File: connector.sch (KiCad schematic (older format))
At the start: 2 parts, among them J11 Conn_02x05_Counter_Clockwise, J12 DB9_Male_MountingHoles

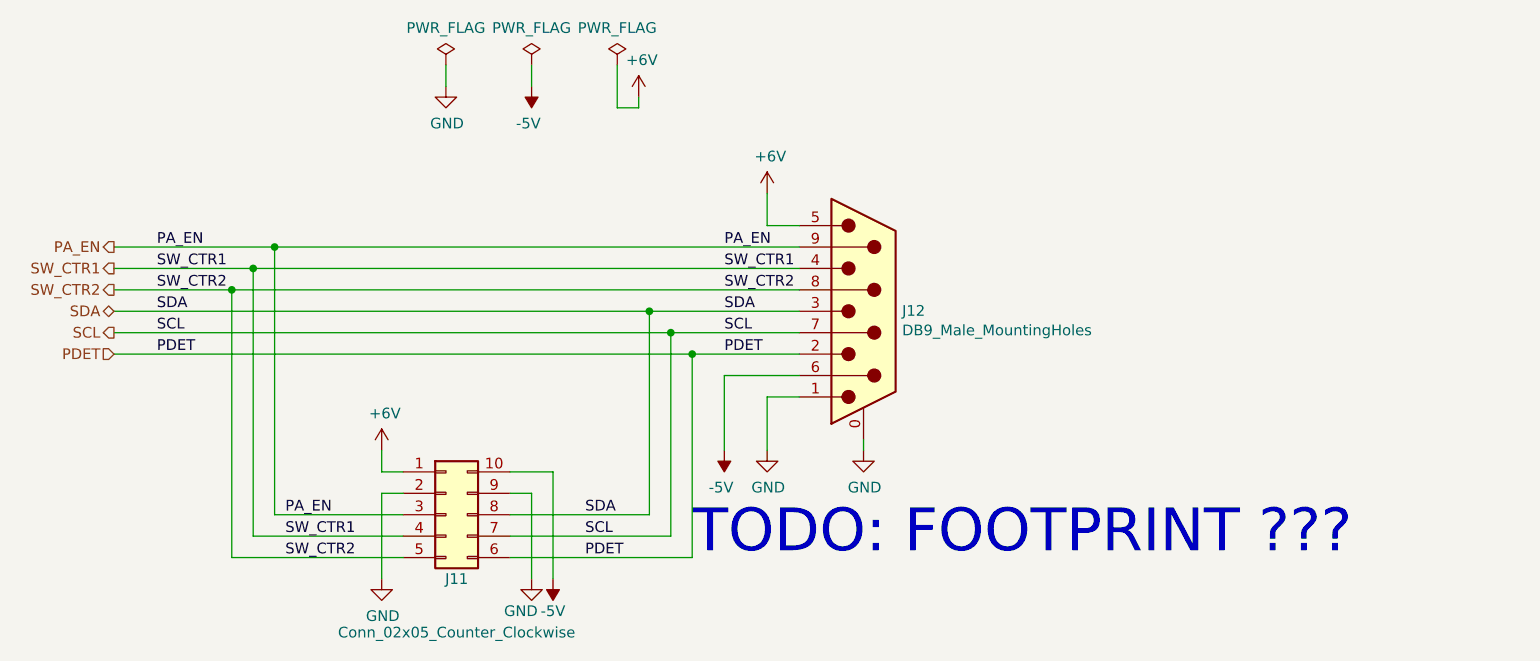
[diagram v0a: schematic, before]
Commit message: First layout
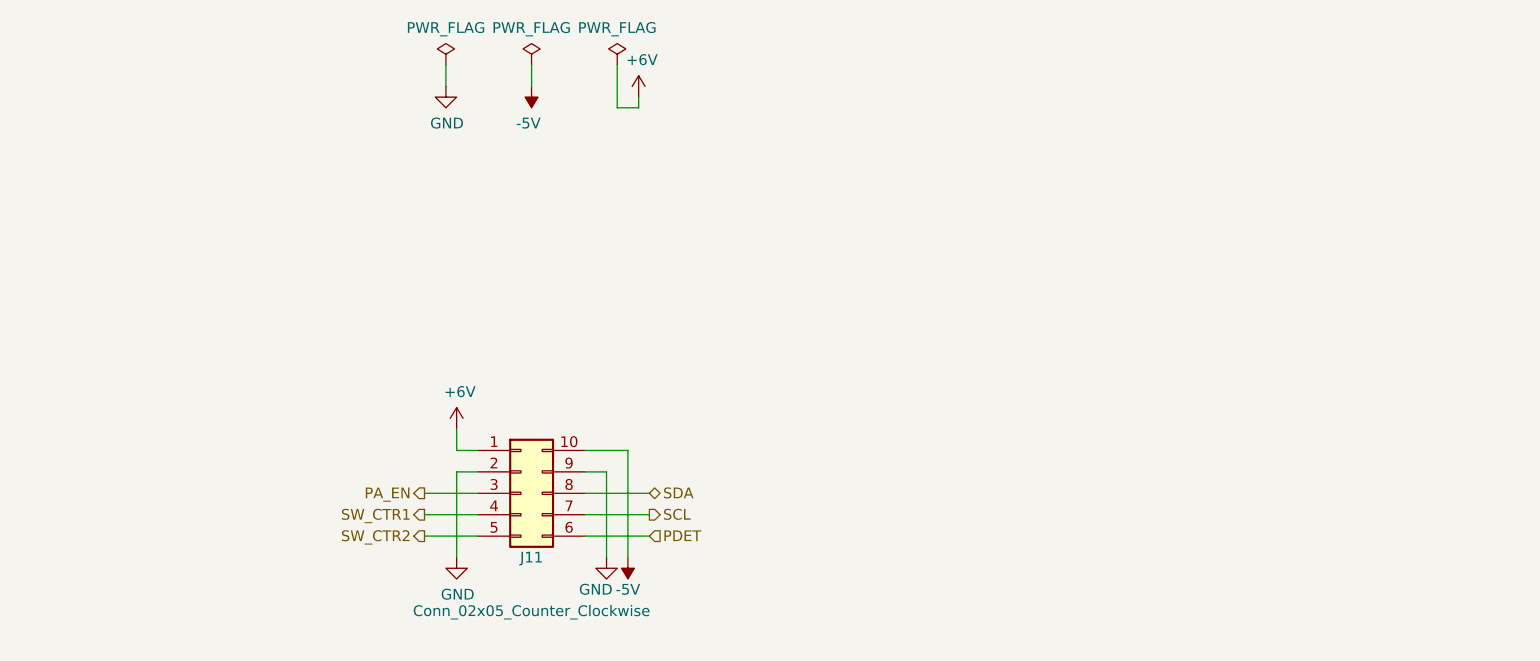
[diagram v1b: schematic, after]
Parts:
- removed J12: DB9_Male_MountingHoles, symbol Connector:DB9_Male_MountingHoles
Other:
- note removed: "TODO: FOOTPRINT ???\n"
- moved on the sheet: J11

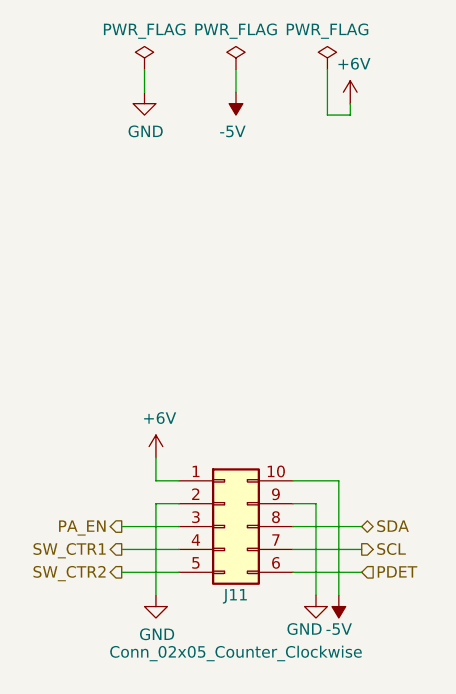
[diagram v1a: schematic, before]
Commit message: Fixed connector
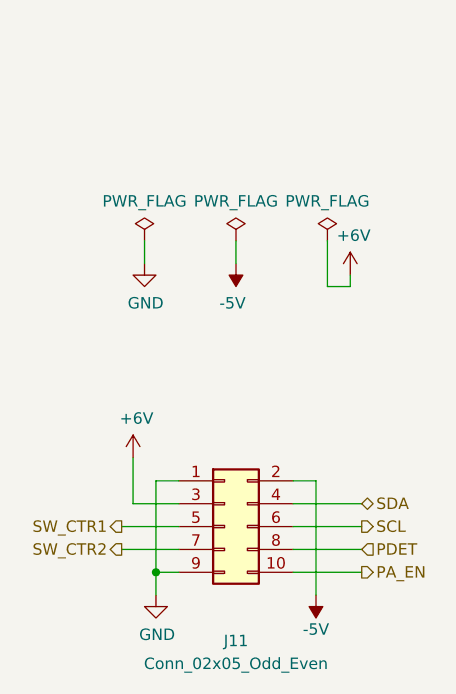
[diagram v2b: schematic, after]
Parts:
- removed J11: Conn_02x05_Counter_Clockwise, Connector_IDC:IDC-Header_2x05_P2.54mm_Vertical, symbol Connector_Generic:Conn_02x05_Counter_Clockwise
- added J11: Conn_02x05_Odd_Even, Connector_IDC:IDC-Header_2x05_P2.54mm_Vertical, symbol Connector_Generic:Conn_02x05_Odd_Even
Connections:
- net +6V: now also J11.3 (Pin_3)
- net -5V: now also J11.2 (Pin_2)
- net GND: now also J11.1 (Pin_1), J11.9 (Pin_9)
- net PA_EN: now also J11.10 (Pin_10)
- net PDET: now also J11.8 (Pin_8)
- net SCL: now also J11.6 (Pin_6)
- net SDA: now also J11.4 (Pin_4)
- net SW_CTR1: now also J11.5 (Pin_5)
- net SW_CTR2: now also J11.7 (Pin_7)
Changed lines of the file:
@@
 Comment4 ""
 $EndDescr
+Text HLabel 6300 4450 2    50   Output ~ 0
+PA_EN
 Text HLabel 5250 4250 0    50   Output ~ 0
-PA_EN
+SW_CTR1
 Text HLabel 5250 4350 0    50   Output ~ 0
-SW_CTR1
-Text HLabel 5250 4450 0    50   Output ~ 0
 SW_CTR2
-Text HLabel 6300 4250 2    50   BiDi ~ 0
+Text HLabel 6300 4150 2    50   BiDi ~ 0
 SDA
-Text HLabel 6300 4350 2    50   Output ~ 0
+Text HLabel 6300 4250 2    50   Output ~ 0
 SCL
-Text HLabel 6300 4450 2    50   Input ~ 0
+Text HLabel 6300 4350 2    50   Input ~ 0
 PDET
 $Comp
 L power:GND #PWR0109
 U 1 1 606566FC
-P 5350 2350
-F 0 "#PWR0109" H 5350 2100 50  0001 C CNN
-F 1 "GND" H 5355 2177 50  0000 C CNN
-F 2 "" H 5350 2350 50  0001 C CNN
-F 3 "" H 5350 2350 50  0001 C CNN
-	1    5350 2350
+P 5350 3100
+F 0 "#PWR0109" H 5350 2850 50  0001 C CNN
+F 1 "GND" H 5355 2927 50  0000 C CNN
+F 2 "" H 5350 3100 50  0001 C CNN
+F 3 "" H 5350 3100 50  0001 C CNN
+	1    5350 3100
 	1    0    0    -1
 $EndComp
@@
 L power:PWR_FLAG #FLG0101
 U 1 1 60656A1B
-P 5350 2250
-F 0 "#FLG0101" H 5350 2325 50  0001 C CNN
-F 1 "PWR_FLAG" H 5350 2423 50  0000 C CNN
-F 2 "" H 5350 2250 50  0001 C CNN
-F 3 "~" H 5350 2250 50  0001 C CNN
-	1    5350 2250
+P 5350 3000
+F 0 "#FLG0101" H 5350 3075 50  0001 C CNN
+F 1 "PWR_FLAG" H 5350 3173 50  0000 C CNN
+F 2 "" H 5350 3000 50  0001 C CNN
+F 3 "~" H 5350 3000 50  0001 C CNN
+	1    5350 3000
 	1    0    0    -1
 $EndComp
 Wire Wire Line
-	5350 2250 5350 2350
+	5350 3000 5350 3100
 $Comp
 L power:-5V #PWR0110
 U 1 1 60656FB7
-P 5750 2350
-F 0 "#PWR0110" H 5750 2450 50  0001 C CNN
-F 1 "-5V" H 5765 2523 50  0000 C CNN
-F 2 "" H 5750 2350 50  0001 C CNN
-F 3 "" H 5750 2350 50  0001 C CNN
-	1    5750 2350
+P 5750 3100
+F 0 "#PWR0110" H 5750 3200 50  0001 C CNN
+F 1 "-5V" H 5765 3273 50  0000 C CNN
+F 2 "" H 5750 3100 50  0001 C CNN
+F 3 "" H 5750 3100 50  0001 C CNN
+	1    5750 3100
 	-1   0    0    1
 $EndComp
@@
 L power:PWR_FLAG #FLG0102
 U 1 1 60657391
-P 5750 2250
-F 0 "#FLG0102" H 5750 2325 50  0001 C CNN
-F 1 "PWR_FLAG" H 5750 2423 50  0000 C CNN
-F 2 "" H 5750 2250 50  0001 C CNN
-F 3 "~" H 5750 2250 50  0001 C CNN
-	1    5750 2250
+P 5750 3000
+F 0 "#FLG0102" H 5750 3075 50  0001 C CNN
+F 1 "PWR_FLAG" H 5750 3173 50  0000 C CNN
+F 2 "" H 5750 3000 50  0001 C CNN
+F 3 "~" H 5750 3000 50  0001 C CNN
+	1    5750 3000
 	1    0    0    -1
 $EndComp
 Wire Wire Line
-	5750 2250 5750 2350
+	5750 3000 5750 3100
 $Comp
 L power:+6V #PWR0111
 U 1 1 60657FE5
-P 6250 2400
-F 0 "#PWR0111" H 6250 2250 50  0001 C CNN
-F 1 "+6V" H 6265 2573 50  0000 C CNN
-F 2 "" H 6250 2400 50  0001 C CNN
-F 3 "" H 6250 2400 50  0001 C CNN
-	1    6250 2400
+P 6250 3150
+F 0 "#PWR0111" H 6250 3000 50  0001 C CNN
+F 1 "+6V" H 6265 3323 50  0000 C CNN
+F 2 "" H 6250 3150 50  0001 C CNN
+F 3 "" H 6250 3150 50  0001 C CNN
+	1    6250 3150
 	1    0    0    -1
 $EndComp
@@
 L power:PWR_FLAG #FLG0103
 U 1 1 60658429
-P 6150 2250
-F 0 "#FLG0103" H 6150 2325 50  0001 C CNN
-F 1 "PWR_FLAG" H 6150 2423 50  0000 C CNN
-F 2 "" H 6150 2250 50  0001 C CNN
-F 3 "~" H 6150 2250 50  0001 C CNN
-	1    6150 2250
+P 6150 3000
+F 0 "#FLG0103" H 6150 3075 50  0001 C CNN
+F 1 "PWR_FLAG" H 6150 3173 50  0000 C CNN
+F 2 "" H 6150 3000 50  0001 C CNN
+F 3 "~" H 6150 3000 50  0001 C CNN
+	1    6150 3000
 	1    0    0    -1
 $EndComp
 Wire Wire Line
-	6150 2250 6150 2450
+	6150 3000 6150 3200
 Wire Wire Line
-	6150 2450 6250 2450
+	6150 3200 6250 3200
 Wire Wire Line
-	6250 2450 6250 2400
-$Comp
-L Connector_Generic:Conn_02x05_Counter_Clockwise J11
-U 1 1 606A85A2
-P 5700 4250
-F 0 "J11" H 5750 3950 50  0000 C CNN
-F 1 "Conn_02x05_Counter_Clockwise" H 5750 3700 50  0000 C CNN
-F 2 "Connector_IDC:IDC-Header_2x05_P2.54mm_Vertical" H 5700 4250 50  0001 C CNN
-F 3 "~" H 5700 4250 50  0001 C CNN
-	1    5700 4250
-	1    0    0    -1
-$EndComp
+	6250 3200 6250 3150
+Wire Wire Line
+	6000 4250 6300 4250
 Wire Wire Line
 	6000 4350 6300 4350
-Wire Wire Line
-	6000 4450 6300 4450
 $Comp
 L power:+6V #PWR0107
 U 1 1 606E1715
-P 5400 3950
-F 0 "#PWR0107" H 5400 3800 50  0001 C CNN
-F 1 "+6V" H 5415 4123 50  0000 C CNN
-F 2 "" H 5400 3950 50  0001 C CNN
-F 3 "" H 5400 3950 50  0001 C CNN
-	1    5400 3950
+P 5300 3950
+F 0 "#PWR0107" H 5300 3800 50  0001 C CNN
+F 1 "+6V" H 5315 4123 50  0000 C CNN
+F 2 "" H 5300 3950 50  0001 C CNN
+F 3 "" H 5300 3950 50  0001 C CNN
+	1    5300 3950
 	1    0    0    -1
 $EndComp
-Wire Wire Line
-	5400 3950 5400 4050
-Wire Wire Line
-	5400 4050 5500 4050
 $Comp
 L power:GND #PWR0108
@@
 	1    0    0    -1
 $EndComp
-Wire Wire Line
-	5400 4550 5400 4150
-Wire Wire Line
-	5400 4150 5500 4150
 $Comp
 L power:-5V #PWR0112
 U 1 1 606E3CEE
-P 6200 4550
-F 0 "#PWR0112" H 6200 4650 50  0001 C CNN
-F 1 "-5V" H 6200 4700 50  0000 C CNN
-F 2 "" H 6200 4550 50  0001 C CNN
-F 3 "" H 6200 4550 50  0001 C CNN
-	1    6200 4550
-	-1   0    0    1
-$EndComp
-$Comp
-L power:GND #PWR0113
-U 1 1 606E4A32
 P 6100 4550
-F 0 "#PWR0113" H 6100 4300 50  0001 C CNN
-F 1 "GND" H 6050 4400 50  0000 C CNN
+F 0 "#PWR0112" H 6100 4650 50  0001 C CNN
+F 1 "-5V" H 6100 4700 50  0000 C CNN
 F 2 "" H 6100 4550 50  0001 C CNN
 F 3 "" H 6100 4550 50  0001 C CNN
 	1    6100 4550
-	1    0    0    -1
+	-1   0    0    1
 $EndComp
-Wire Wire Line
-	6100 4550 6100 4150
-Wire Wire Line
-	6100 4150 6000 4150
-Wire Wire Line
-	6200 4550 6200 4050
-Wire Wire Line
-	6200 4050 6000 4050
 Wire Wire Line
 	5250 4250 5500 4250
@@
 	5250 4350 5500 4350
 Wire Wire Line
-	5250 4450 5500 4450
+	6300 4450 6000 4450
 Wire Wire Line
-	6000 4250 6300 4250
+	6000 4150 6300 4150
+Wire Wire Line
+	5400 4050 5500 4050
+Wire Wire Line
+	5400 4050 5400 4450
+Wire Wire Line
+	5300 3950 5300 4150
+$Comp
+L Connector_Generic:Conn_02x05_Odd_Even J11
+U 1 1 6067C933
+P 5700 4250
+F 0 "J11" H 5750 3750 50  0000 C CNN
+F 1 "Conn_02x05_Odd_Even" H 5750 3650 50  0000 C CNN
+F 2 "Connector_IDC:IDC-Header_2x05_P2.54mm_Vertical" H 5700 4250 50  0001 C CNN
+F 3 "~" H 5700 4250 50  0001 C CNN
+	1    5700 4250
+	1    0    0    -1
+$EndComp
+Wire Wire Line
+	5300 4150 5500 4150
+Wire Wire Line
+	5500 4450 5400 4450
+Connection ~ 5400 4450
+Wire Wire Line
+	5400 4450 5400 4550
+Wire Wire Line
+	6100 4050 6100 4550
+Wire Wire Line
+	6100 4050 6000 4050
 $EndSCHEMATC
